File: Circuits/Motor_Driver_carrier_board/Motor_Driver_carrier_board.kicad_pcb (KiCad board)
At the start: 2 copper layers, 35 x 55.6 mm, 21 parts, among them P2 61301021021

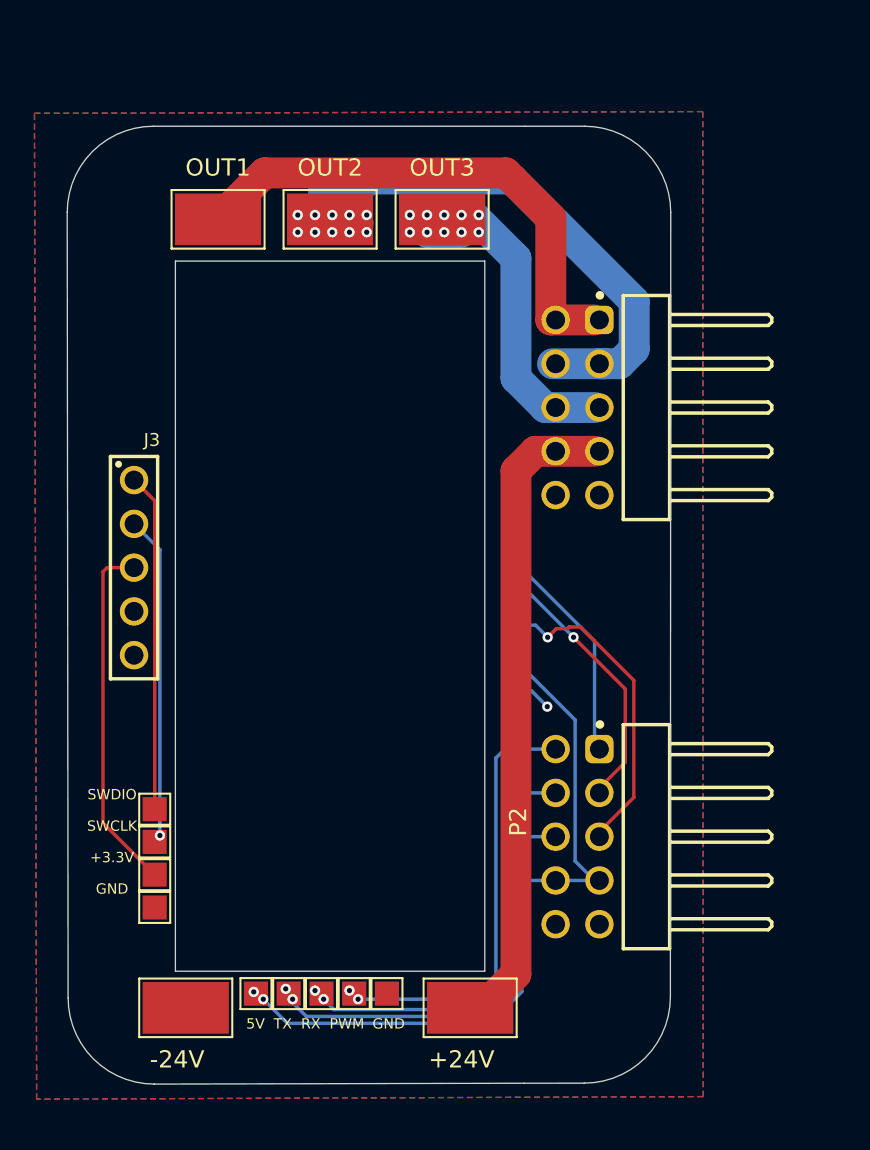
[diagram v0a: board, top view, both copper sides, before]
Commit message: STP to pointer
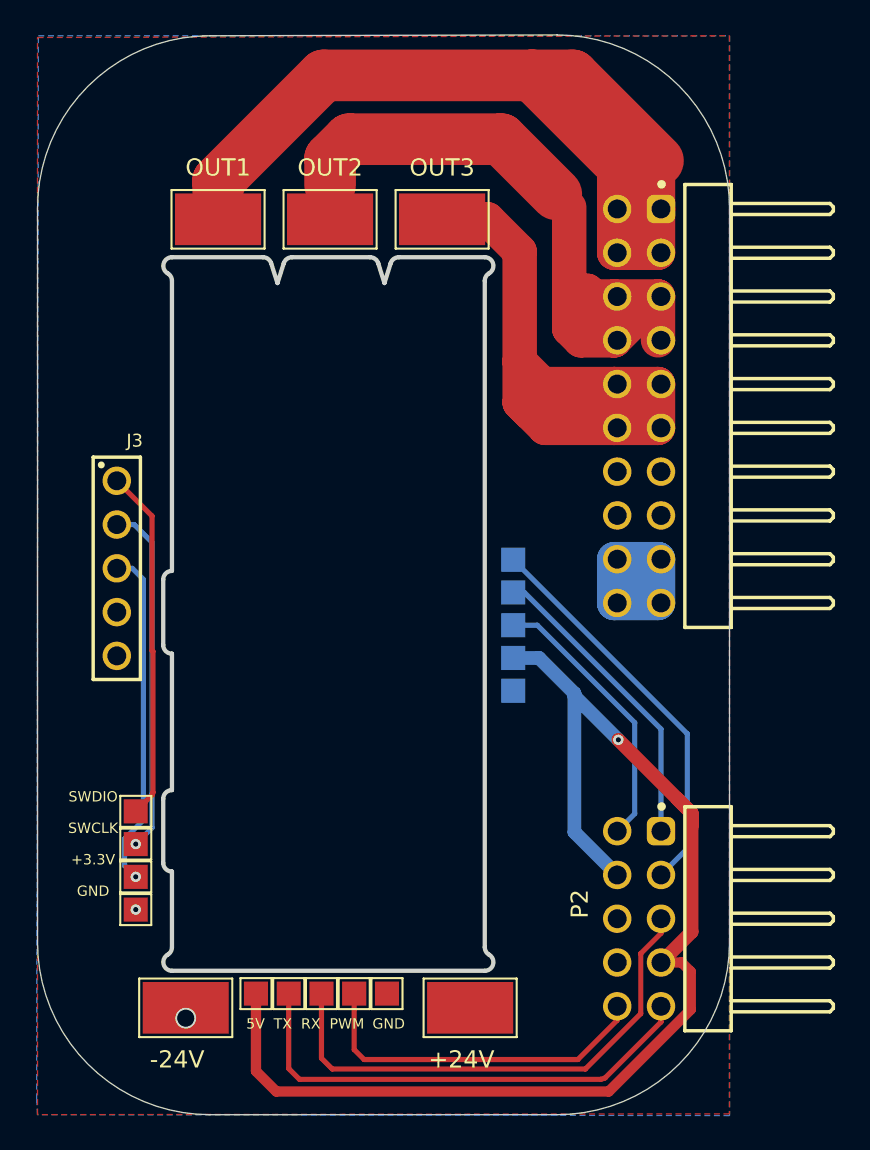
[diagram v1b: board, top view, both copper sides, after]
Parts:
- P2: value 61301021021 -> ESC_Adapter_pins_right_angle; footprint 61301021021:ESC_Adapter_pins_right_angle -> B-G431B-ESC1:ESC_Adapter_pins_right_angle
- moved P2 5.95 mm to (154.8, 74.4)
- moved +3.3V 1.11 mm to (122.9, 85.1)
- moved GND 1.11 mm to (122.9, 87.0)
- moved SWCLK 1.11 mm to (122.9, 83.2)
- moved SWDIO 1.11 mm to (122.9, 81.3)
- moved J3 1.00 mm to (121.8, 67.2)
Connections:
- net /3.3V renamed 3.3V
- net /SWCLK renamed SWCLK
- net /SWDIO renamed SWDIO
- +24V pad 1: /24V -> 24V
- 5V pad 1: /5V -> 5V (x2)
- GND pad 1: GND -> UART_GND
- H1 pad 1: /H1 -> H1
- H2 pad 1: /H2 -> H2
- H3 pad 1: /H3 -> H3
- OUT1 pad 1: /OUT1 -> OUT1
- OUT2 pad 1: /OUT2 -> OUT2
- OUT3 pad 1: /OUT3 -> OUT3
- P2 pad 1: /OUT1 -> OUT1
- P2 pad 10: GND -> OUT3
- P2 pad 11: /H1 -> OUT3
- P2 pad 12: /PWM -> OUT3
- P2 pad 13: /H2 -> 24V
- P2 pad 14: /RX -> 24V
- P2 pad 15: /H3 -> 24V
- P2 pad 16: /TX -> 24V
- P2 pad 17: /5V -> GND
- P2 pad 18: /5V -> GND
- P2 pad 2: /OUT1 -> OUT1
- P2 pad 3: /OUT2 -> OUT1
- P2 pad 4: /OUT2 -> OUT1
- P2 pad 5: /OUT3 -> OUT2
- P2 pad 6: /OUT3 -> OUT2
- P2 pad 7: /24V -> OUT2
- P2 pad 8: /24V -> OUT2
- P2 pad 9: GND -> OUT3
- PWM pad 1: /PWM -> PWM
- RX pad 1: /RX -> RX
- TX pad 1: /TX -> TX
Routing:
- net 5V: track 0.00 -> 73.4 mm, vias 0 -> 1
- net OUT1: track 0.00 -> 60.5 mm
- net OUT3: track 0.00 -> 43.6 mm
- net /5V: track 43.2 -> 0.00 mm, vias 2 -> 0
- net OUT2: track 0.00 -> 42.9 mm
- net /OUT2: track 40.2 -> 0.00 mm, vias 10 -> 0
- net /24V: track 37.7 -> 0.00 mm
- net /OUT1: track 30.0 -> 0.00 mm
- net RX: track 0.00 -> 29.9 mm
- net TX: track 0.00 -> 28.5 mm
- net /TX: track 26.0 -> 0.00 mm, vias 2 -> 0
- net /PWM: track 25.9 -> 0.00 mm, vias 2 -> 0
- net /RX: track 25.9 -> 0.00 mm, vias 2 -> 0
- net H1: track 0.00 -> 23.1 mm
- net /OUT3: track 22.1 -> 0.00 mm, vias 10 -> 0
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- added copper zone on F.Cu, net 24V
- removed copper zone on F.Cu, net GND
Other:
- board size 35 x 55.6 mm -> 40.2 x 62.7 mm
